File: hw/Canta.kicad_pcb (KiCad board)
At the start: 2 copper layers, 85.6 x 54 mm, 36 parts, among them J2 USB_C_Receptacle_USB2.0_14P, SW1 SW_SPST, U1 CH591F, U2 MAX98357A, U3 USBLC6-2SC6, U4 ME6206A33XG, Y1 32MHz

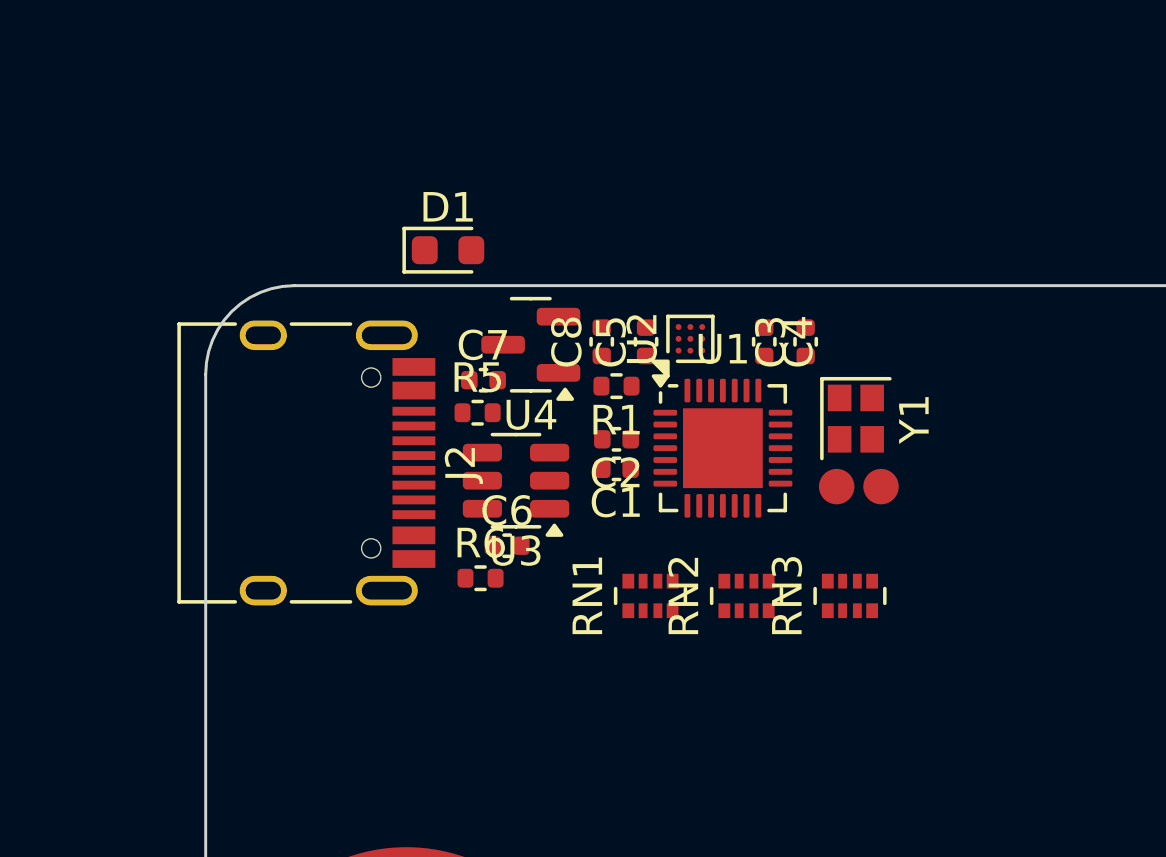
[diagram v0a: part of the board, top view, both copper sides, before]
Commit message: hw: Layout...?
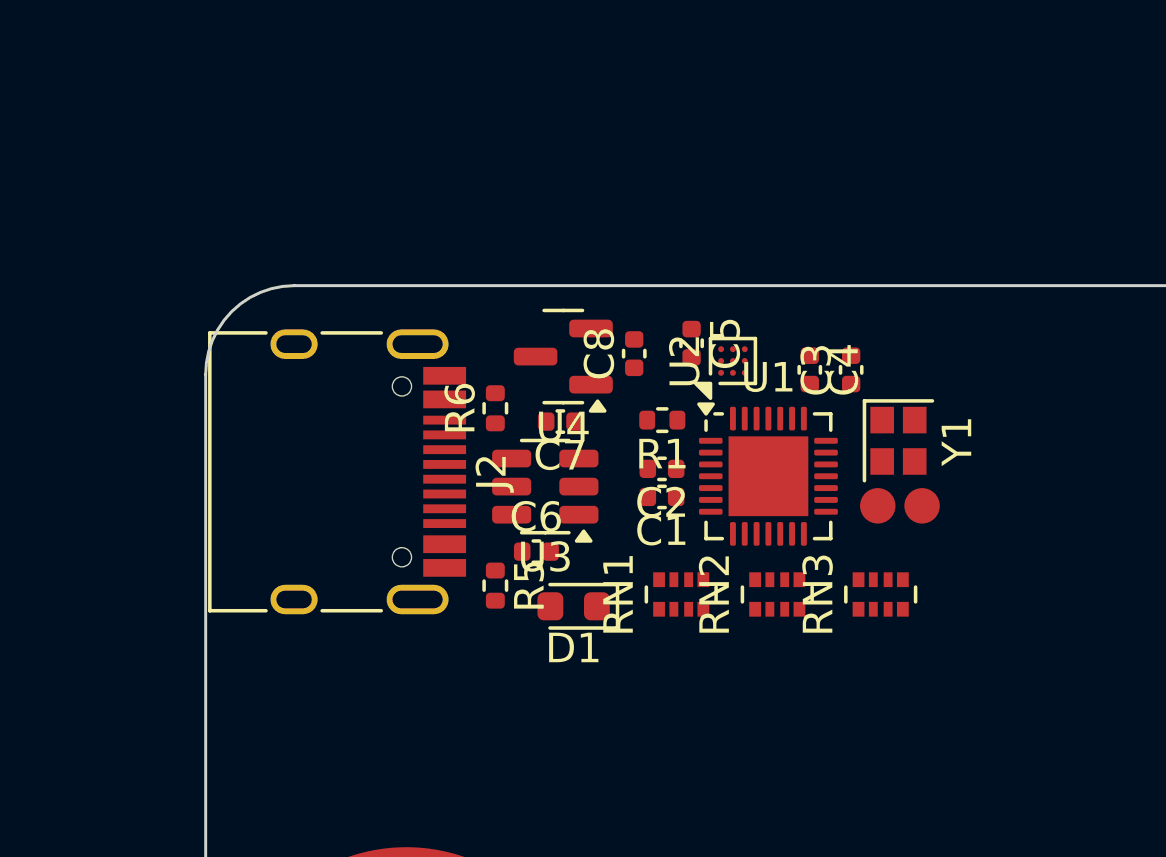
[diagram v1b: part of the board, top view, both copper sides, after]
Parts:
- moved D1 12.8 mm to (62.5, 60.9), turned to 180 degrees
- moved C7 2.95 mm to (62.0, 54.6), turned to 180 degrees
- moved R1 1.93 mm to (65.5, 54.5)
- moved C2 1.84 mm to (65.4, 56.2)
- moved C3 1.81 mm to (71.8, 52.9)
- moved U1 1.81 mm to (69.0, 56.5)
- moved C1 1.81 mm to (65.4, 57.1)
- moved C4 1.81 mm to (70.4, 52.9)
- moved U2 1.62 mm to (67.8, 52.5)
- moved Y1 1.62 mm to (73.4, 55.2)
- moved C5 1.54 mm to (66.4, 52.0), turned to -90 degrees
- moved SW1 1.53 mm to (73.5, 57.5)
- moved C8 1.17 mm to (64.5, 52.3)
- moved U4 1.17 mm to (62.1, 52.4)
- moved J2 1.08 mm to (54.0, 56.3)
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- renumbered R6 to R5, R5 to R6
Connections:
- R5 pad 1: Net-(J2-CC1) -> Net-(J2-CC2)
- R6 pad 1: Net-(J2-CC2) -> Net-(J2-CC1)
